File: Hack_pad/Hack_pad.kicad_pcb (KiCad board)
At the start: 2 copper layers, 42.9 x 82.1 mm, 10 parts, among them SW1 SW_Push, SW2 SW_Push, SW3 SW_Push, SW4 SW_Push, SW5 RotaryEncoder_Switch, U1 XIAO-RP2040-DIP

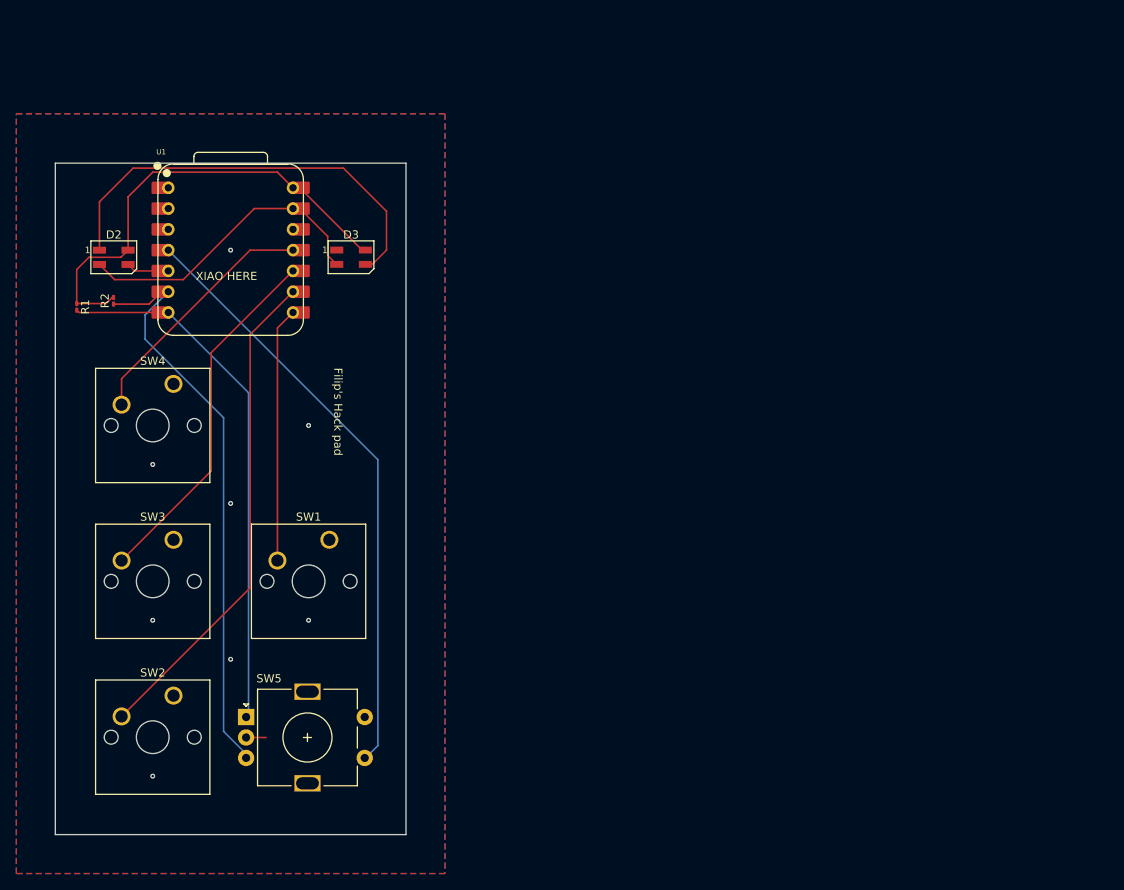
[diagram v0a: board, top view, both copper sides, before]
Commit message: update
recrated
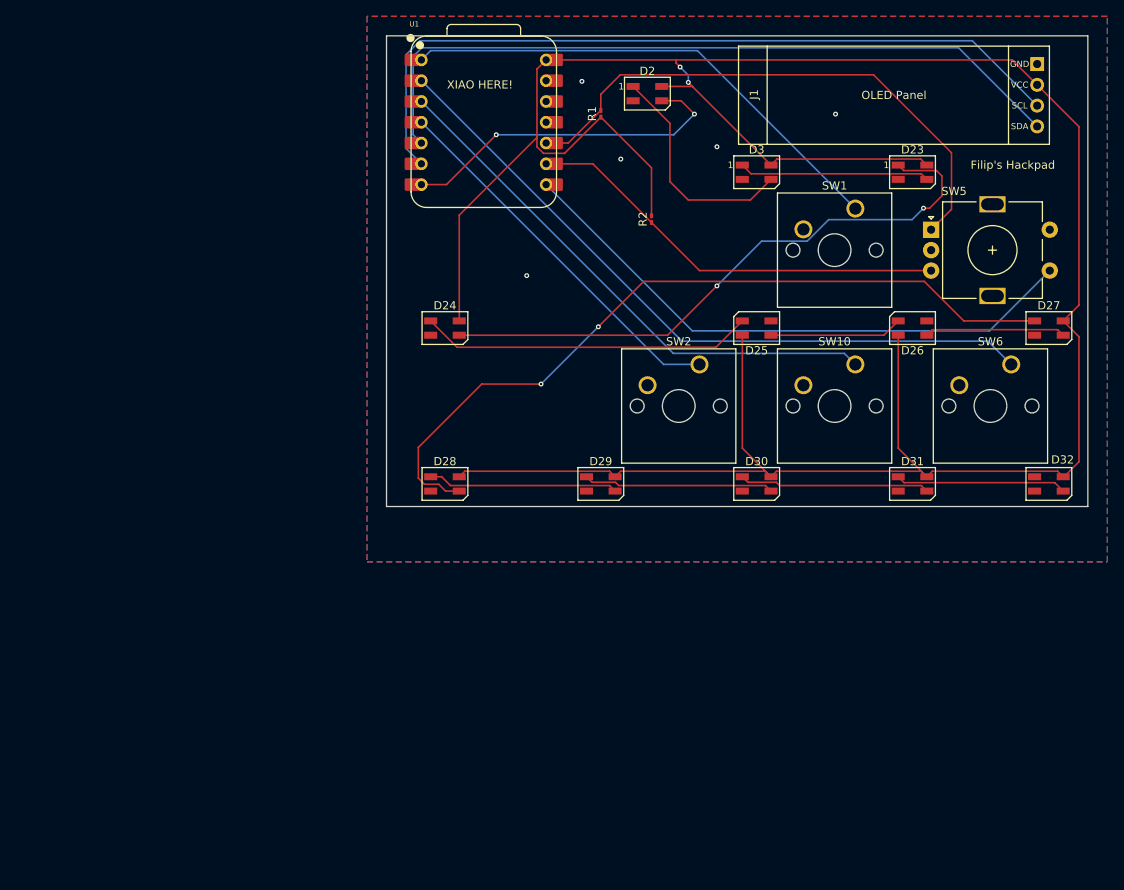
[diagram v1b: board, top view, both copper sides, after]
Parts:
- removed SW3, SW4: SW_Push, Button_Switch_Keyboard:SW_Cherry_MX_1.00u_PCB
- added D23: SK6812MINI, LED_SMD:LED_SK6812MINI_PLCC4_3.5x3.5mm_P1.75mm, F.Cu at (202.4, 88.1)
- added D24: SK6812MINI, LED_SMD:LED_SK6812MINI_PLCC4_3.5x3.5mm_P1.75mm, F.Cu at (145.3, 107.2)
- added D25: SK6812MINI, LED_SMD:LED_SK6812MINI_PLCC4_3.5x3.5mm_P1.75mm, F.Cu at (183.4, 107.2)
- added D26: SK6812MINI, LED_SMD:LED_SK6812MINI_PLCC4_3.5x3.5mm_P1.75mm, F.Cu at (202.4, 107.2)
- added D27: SK6812MINI, LED_SMD:LED_SK6812MINI_PLCC4_3.5x3.5mm_P1.75mm, F.Cu at (219.1, 107.2)
- added D28: SK6812MINI, LED_SMD:LED_SK6812MINI_PLCC4_3.5x3.5mm_P1.75mm, F.Cu at (145.3, 126.2)
- added D29: SK6812MINI, LED_SMD:LED_SK6812MINI_PLCC4_3.5x3.5mm_P1.75mm, F.Cu at (164.3, 126.2)
- added D30: SK6812MINI, LED_SMD:LED_SK6812MINI_PLCC4_3.5x3.5mm_P1.75mm, F.Cu at (183.4, 126.2)
- added D31: SK6812MINI, LED_SMD:LED_SK6812MINI_PLCC4_3.5x3.5mm_P1.75mm, F.Cu at (202.4, 126.2)
- added D32: SK6812MINI, LED_SMD:LED_SK6812MINI_PLCC4_3.5x3.5mm_P1.75mm, F.Cu at (219.1, 126.2)
- added J1: Oled, oled:SSD1306-0.91-OLED-4pin-128x32, F.Cu at (181.1, 72.7)
- added SW10: SW_Push, Button_Switch_Keyboard:SW_Cherry_MX_1.00u_PCB, F.Cu at (195.4, 111.6)
- added SW6: SW_Push, Button_Switch_Keyboard:SW_Cherry_MX_1.00u_PCB, F.Cu at (214.5, 111.6)
- moved SW5 102.8 mm to (204.7, 95.1)
- moved SW2 76.0 mm to (176.4, 111.6)
- moved SW1 76.0 mm to (195.4, 92.6)
- moved R1 68.3 mm to (164.3, 81.0), turned to 90 degrees
- moved D2 68.2 mm to (170.0, 78.5)
- moved R2 66.5 mm to (170.5, 93.8)
- moved D3 50.7 mm to (183.4, 88.1)
- moved U1 34.7 mm to (150.0, 82.0)
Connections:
- D3 pad 1: unconnected-(D3-DOUT-Pad1) -> Net-(D23-DIN)
- R1 pad 2: Net-(U1-GPIO0/TX) -> Net-(U1-GPIO4/MISO)
- R2 pad 1: Net-(U1-GPIO7/SCL) -> Net-(U1-GPIO2/SCK)
- SW1 pad 1: GND -> Net-(U1-GPIO26/ADC0/A0)
- SW1 pad 2: Net-(U1-GPIO1/RX) -> GND
- SW2 pad 1: GND -> Net-(U1-GPIO29/ADC3/A3)
- SW2 pad 2: Net-(U1-GPIO2/SCK) -> GND
- SW5 pad A: Net-(U1-GPIO0/TX) -> Net-(U1-GPIO4/MISO)
- SW5 pad B: Net-(U1-GPIO7/SCL) -> Net-(U1-GPIO2/SCK)
- SW5 pad S1: Net-(U1-GPIO29/ADC3/A3) -> Net-(U1-GPIO1/RX)
- U1 pad 1: unconnected-(U1-GPIO26/ADC0/A0-Pad1) -> Net-(U1-GPIO26/ADC0/A0)
- U1 pad 11: Net-(U1-GPIO3/MOSI) -> unconnected-(U1-GPIO3/MOSI-Pad11)
- U1 pad 2: unconnected-(U1-GPIO27/ADC1/A1-Pad2) -> Net-(U1-GPIO27/ADC1/A1)
- U1 pad 3: unconnected-(U1-GPIO28/ADC2/A2-Pad3) -> Net-(U1-GPIO28/ADC2/A2)
- U1 pad 5: Net-(D2-DIN) -> Net-(J1-Pin_4)
- U1 pad 6: Net-(U1-GPIO7/SCL) -> Net-(J1-Pin_3)
- U1 pad 7: Net-(U1-GPIO0/TX) -> Net-(D2-DIN)
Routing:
- net +5V: track 56.1 -> 330.6 mm, vias 0 -> 2
- net Net-(J1-Pin_3): track 0.00 -> 95.2 mm
- net Net-(D27-DOUT): track 0.00 -> 95.1 mm, vias 0 -> 2
- net Net-(J1-Pin_4): track 0.00 -> 91.7 mm
- net Net-(U1-GPIO27/ADC1/A1): track 0.00 -> 86.5 mm
- net Net-(D23-DOUT): track 0.00 -> 74.4 mm, vias 0 -> 2
- net Net-(U1-GPIO7/SCL): track 69.7 -> 0.00 mm
- net Net-(U1-GPIO28/ADC2/A2): track 0.00 -> 66.4 mm
- net Net-(U1-GPIO0/TX): track 63.8 -> 0.00 mm
- net Net-(U1-GPIO26/ADC0/A0): track 0.00 -> 61.5 mm
- net Net-(U1-GPIO1/RX): track 31.1 -> 72.0 mm
- net Net-(D24-DOUT): track 0.00 -> 40.8 mm
- net GND: track 39.2 -> 0.00 mm, vias 0 -> 5
- net Net-(D2-DIN): track 4.41 -> 41.6 mm, vias 0 -> 2
- net Net-(U1-GPIO3/MOSI): track 30.6 -> 0.00 mm
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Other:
- board size 42.9 x 82.1 mm -> 85.7 x 57.5 mm
- board text added: "Filip's Hackpad"
- board text added: "XIAO HERE!"
- board text removed: "Filip's Hack pad"
- board text removed: "XIAO HERE"
